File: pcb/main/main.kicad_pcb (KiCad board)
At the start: 2 copper layers, 29.4 x 98.3 mm, 54 parts, among them J1 Conn_01x04, J2 USB_B, J3 Serial, J4 STLink, J5 RJ45, J6 SELECT, J7 READ, J8 TRACKBALL, SW5 RST_SW, SW6 BOOT0, SW7 BOOT1, U1 3.3v regul, U2 STM32F103C8Tx, Y1 32.768kHz, Y2 8MHz

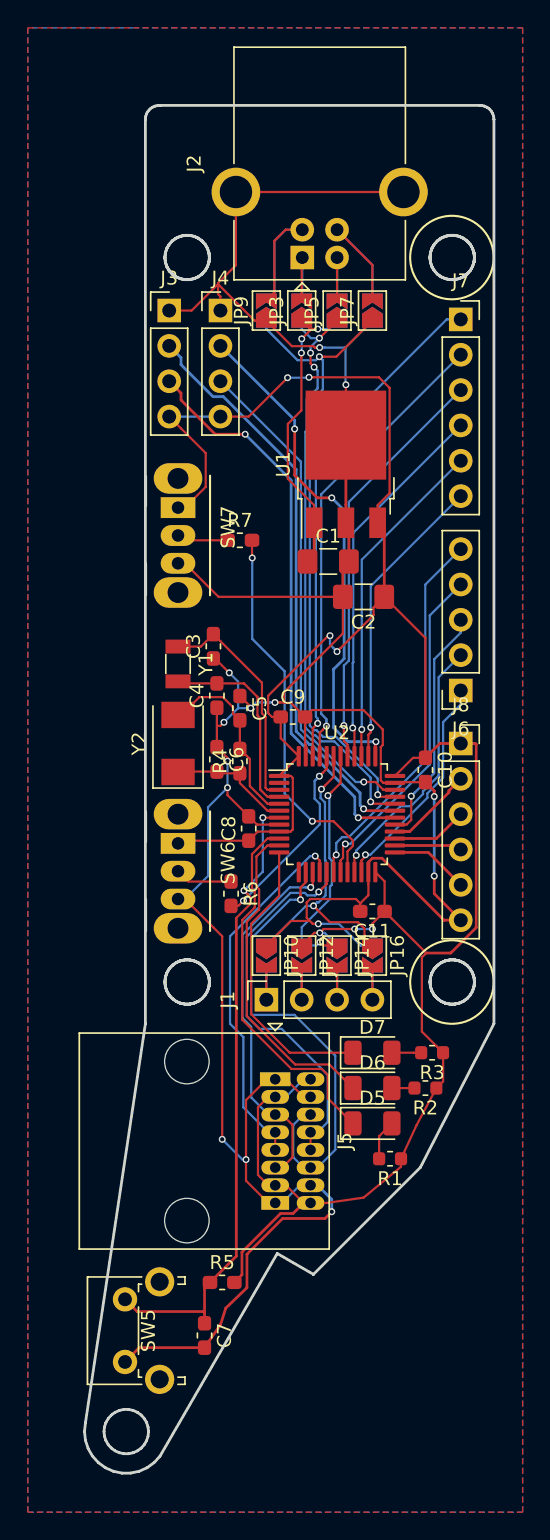
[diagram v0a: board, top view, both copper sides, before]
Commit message: production pcb
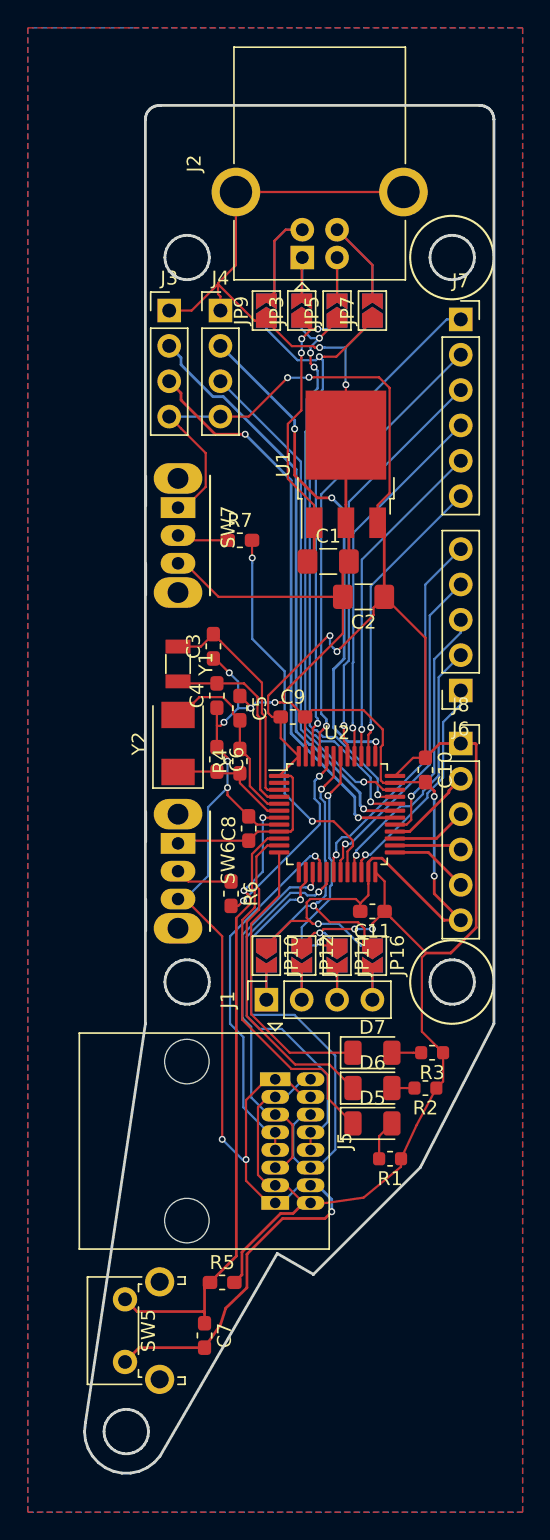
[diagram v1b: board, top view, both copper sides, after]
